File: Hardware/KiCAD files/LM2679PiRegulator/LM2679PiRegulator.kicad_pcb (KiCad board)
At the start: 2 copper layers, 48 x 48 mm, 14 parts, among them J2 Conn_01x03_Pin, U1 LM2679SX-5V

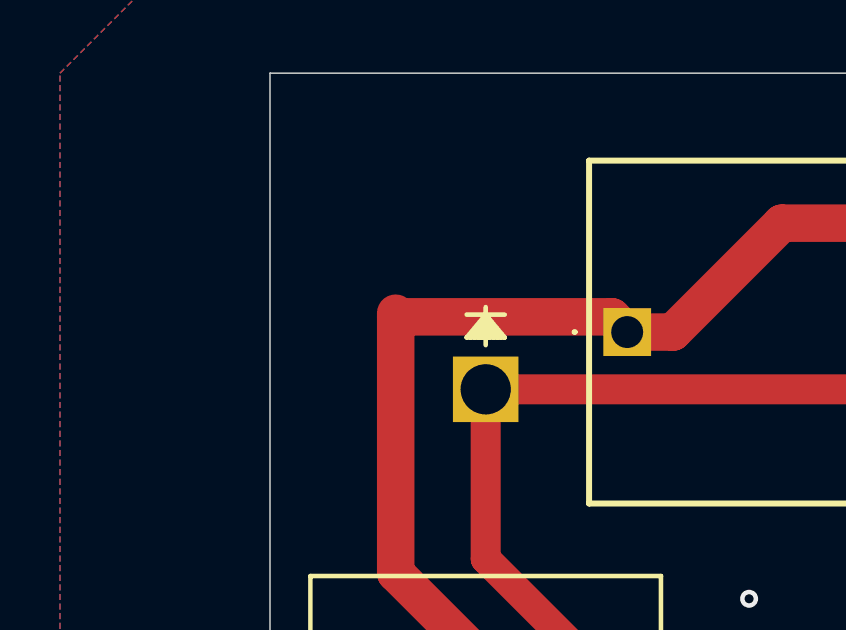
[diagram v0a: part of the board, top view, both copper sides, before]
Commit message: Most recent changes to final submission
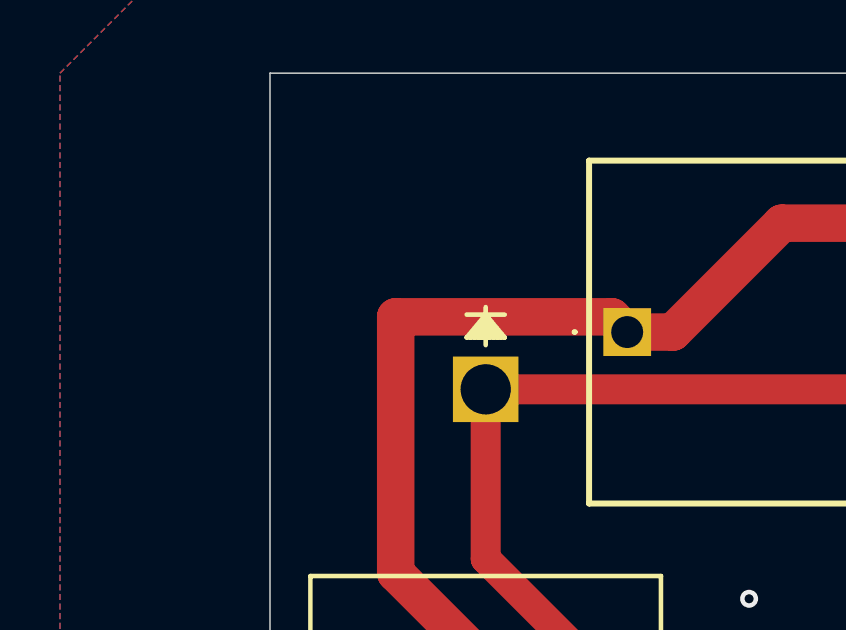
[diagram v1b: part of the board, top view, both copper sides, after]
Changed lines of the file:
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@@
-	)
-	(segment
-		(start 129.19 87.122)
-		(end 129.19 87)
-		(width 1.25)
-		(layer "F.Cu")
-		(net "/Vout")
 	)
 	(segment
